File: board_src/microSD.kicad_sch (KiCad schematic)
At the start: 4 parts, among them IC4 LM317T, J12 112J-TDAR-R01, J14 Conn_01x07

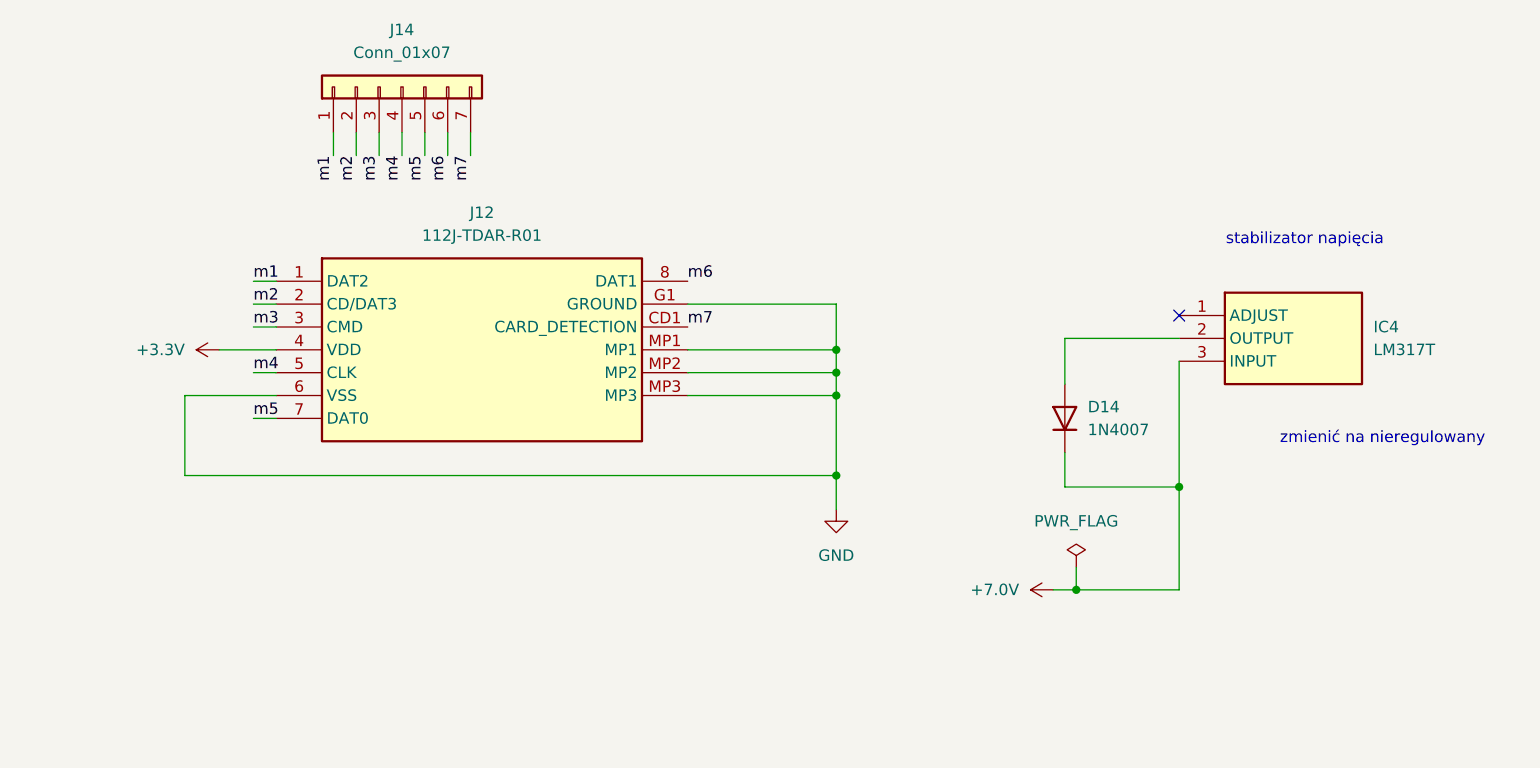
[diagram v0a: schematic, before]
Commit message: uporzadkowane 3D
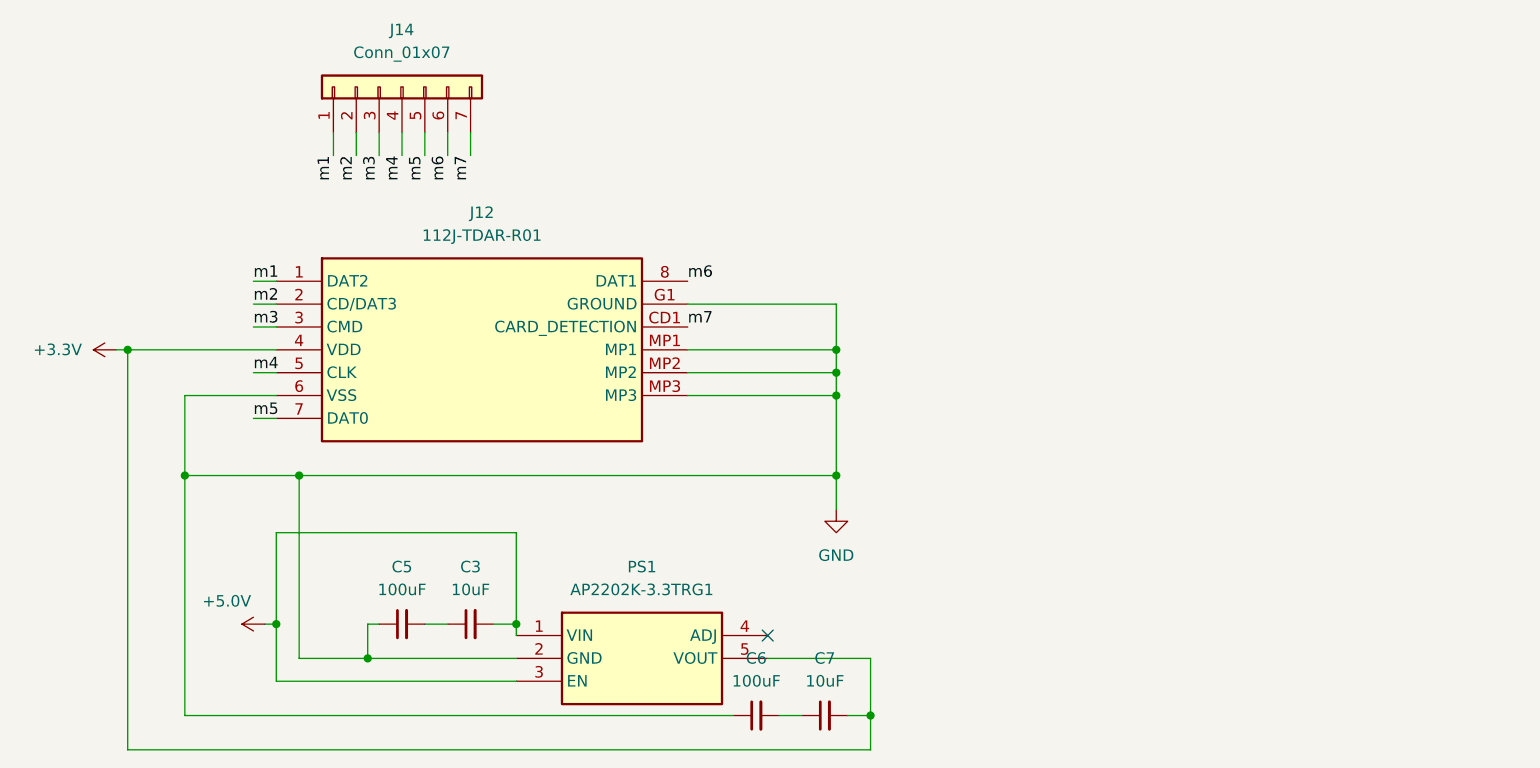
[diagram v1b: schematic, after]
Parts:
- removed D14: 1N4007, Diode_THT:D_DO-41_SOD81_P10.16mm_Horizontal, symbol Diode:1N4007
- removed IC4: LM317T, footprints:TO255P460X1020X2008-3P, symbol LM317T:LM317T
- added C3, C7: 10uF, symbol Device:C_Small
- added C5, C6: 100uF, symbol Device:C_Small
- added PS1: AP2202K-3.3TRG1, footprints:SOT95P282X145-5N, symbol AP2202K-3_3TRG1:AP2202K-3.3TRG1
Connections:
- net +3.3V: now also C7.2, PS1.5 (VOUT)
- net GND: now also C5.1, C6.1, PS1.2 (GND)
- new net: C3.1, C5.2
- new net: C6.2, C7.1
- new net +5.0V: C3.2, PS1.1 (VIN), PS1.3 (EN)
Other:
- note removed: "stabilizator napięcia"
- note removed: "zmienić na nieregulowany"
